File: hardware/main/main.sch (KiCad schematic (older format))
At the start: 2 parts, among them J1 Conn_02x11_Odd_Even, J2 Conn_02x11_Odd_Even

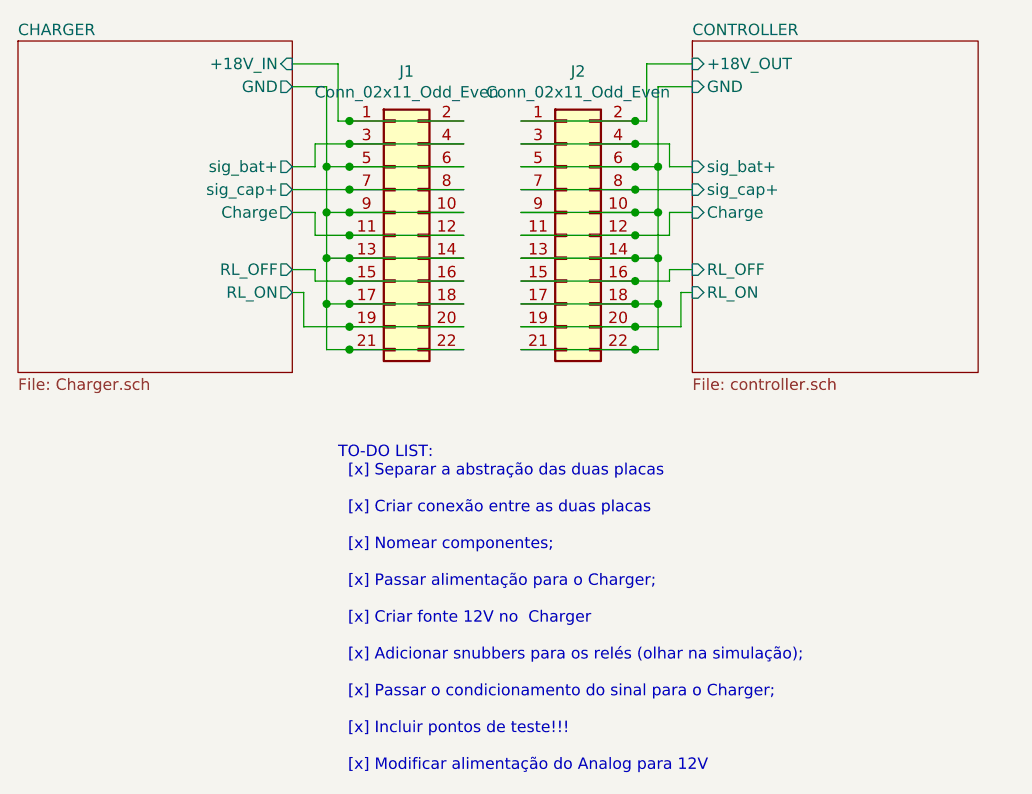
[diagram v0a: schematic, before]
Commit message: Layout retrabalhado. Não finalizado.
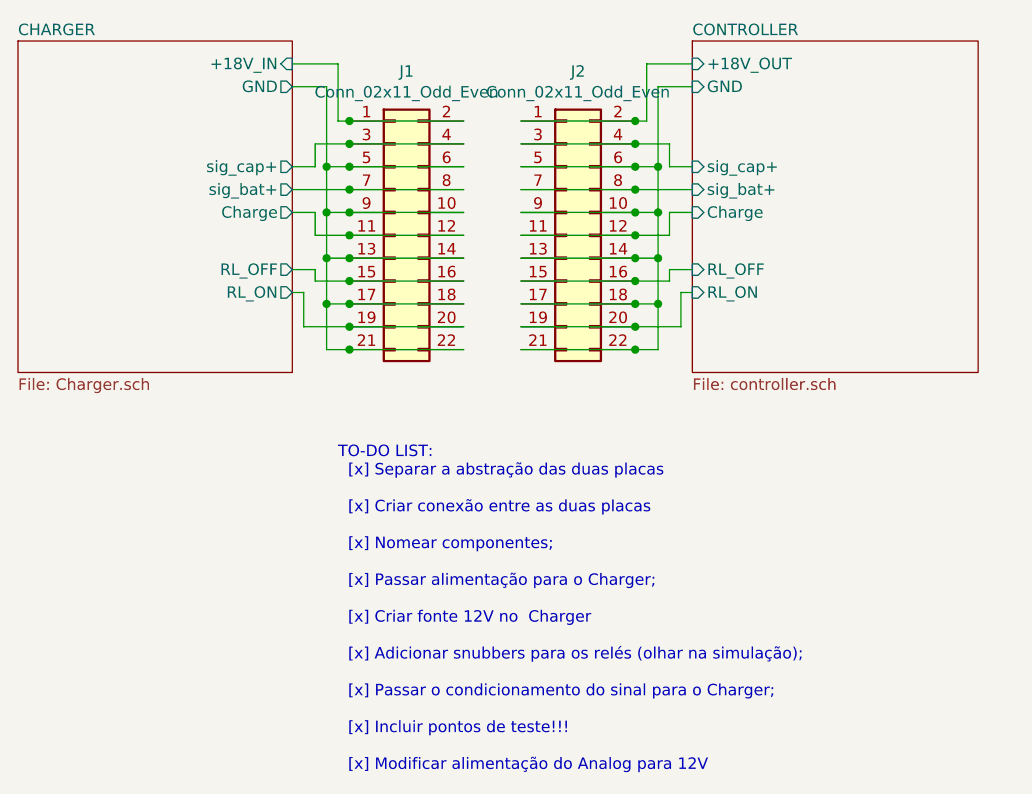
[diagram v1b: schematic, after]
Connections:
- net CHARGER/sig_bat+: now also J1.7 (Pin_7), J1.8 (Pin_8); no longer J1.3 (Pin_3), J1.4 (Pin_4)
- net CHARGER/sig_cap+: now also J1.3 (Pin_3), J1.4 (Pin_4); no longer J1.7 (Pin_7), J1.8 (Pin_8)
- net CONTROLLER/sig_bat+: now also J2.7 (Pin_7), J2.8 (Pin_8); no longer J2.3 (Pin_3), J2.4 (Pin_4)
- net CONTROLLER/sig_cap+: now also J2.3 (Pin_3), J2.4 (Pin_4); no longer J2.7 (Pin_7), J2.8 (Pin_8)
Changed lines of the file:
@@
 EESchema Schematic File Version 4
 LIBS:main-cache
-EELAYER 26 0
+EELAYER 29 0
 EELAYER END
 $Descr A4 11693 8268
@@
 F5 "GND" O R 4250 2600 50
 F6 "+18V_IN" I R 4250 2500 50
-F7 "sig_bat+" O R 4250 2950 50
-F8 "sig_cap+" O R 4250 3050 50
+F7 "sig_bat+" O R 4250 3050 50
+F8 "sig_cap+" O R 4250 2950 50
 $EndSheet
 $Sheet
@@
 F5 "GND" I L 6000 2600 50
 F6 "+18V_OUT" I L 6000 2500 50
-F7 "sig_bat+" I L 6000 2950 50
-F8 "sig_cap+" I L 6000 3050 50
+F7 "sig_bat+" I L 6000 3050 50
+F8 "sig_cap+" I L 6000 2950 50
 $EndSheet
 Wire Wire Line
